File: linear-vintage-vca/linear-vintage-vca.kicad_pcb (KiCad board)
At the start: 2 copper layers, 50.5 x 110 mm, 51 parts, among them J1 Conn_02x08_Odd_Even, J2 AudioJack2, J3 AudioJack2, J4 AudioJack2, J5 AudioJack2, J6 AudioJack2, J7 AudioJack2, J8 AudioJack2, J9 AudioJack2, Q1 BC556, Q2 BC556, U1 LM13700, U2 TL072, U3 TL072

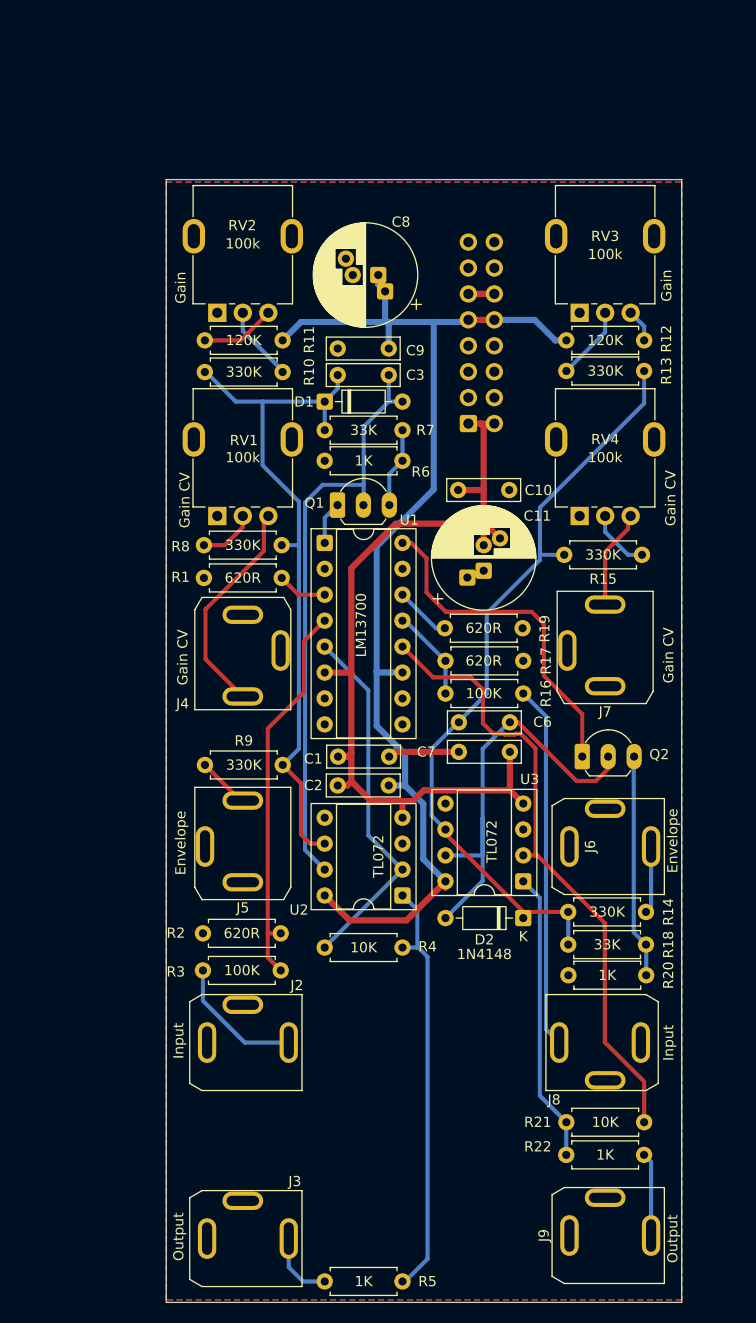
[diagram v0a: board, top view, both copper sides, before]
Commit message: VCA v. 2.0
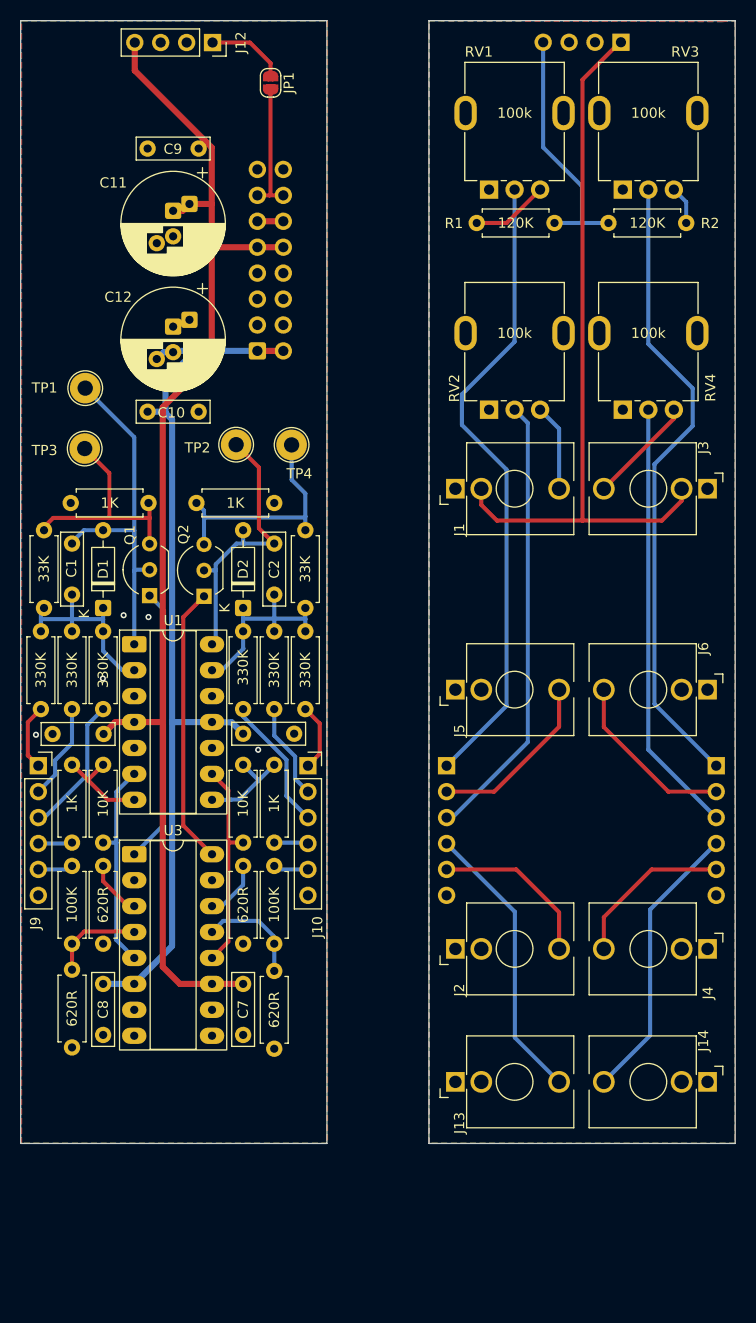
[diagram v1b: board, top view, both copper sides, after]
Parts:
- removed C3: 100n, Capacitor_THT:C_Rect_L7.0mm_W2.0mm_P5.00mm
- removed U2: TL072, Package_DIP:DIP-8_W7.62mm_Socket
- added C12: 47uF, Capacitor_THT:CP_Radial_D10.0mm_P2.50mm_P5.00mm, F.Cu at (50.7, 73.7)
- added C5: 100n, Capacitor_THT:C_Rect_L7.0mm_W2.0mm_P5.00mm, F.Cu at (43.9, 113.6)
- added J10: Conn_01x10_Socket, Connector_PinSocket_2.54mm:PinSocket_1x06_P2.54mm_Vertical, F.Cu at (63.9, 116.7)
- added J11: Conn_01x04_Pin, Connector_PinHeader_2.54mm:PinHeader_1x04_P2.54mm_Vertical, B.Cu at (94.5, 45.8)
- added J12: Conn_01x04_Socket, Connector_PinSocket_2.54mm:PinSocket_1x04_P2.54mm_Vertical, F.Cu at (54.5, 45.8)
- added J13: AudioJack2, linear_vintage_vca:Jack_3.5mm_Switch, F.Cu at (84.1, 147.6)
- added J14: AudioJack2, linear_vintage_vca:Jack_3.5mm_Switch, F.Cu at (97.2, 147.6)
- added J15: Conn_02x08_Odd_Even, Connector_IDC:IDC-Header_2x08_P2.54mm_Vertical, B.Cu at (58.9, 76.0)
- added JP1: SolderJumper_2_Open, Jumper:SolderJumper-2_P1.3mm_Open_RoundedPad1.0x1.5mm, F.Cu at (60.2, 49.8)
- added TP1: TestPoint, TestPoint:TestPoint_Loop_D2.54mm_Drill1.5mm_Beaded, F.Cu at (42.1, 79.7)
- added TP2: TestPoint, TestPoint:TestPoint_Loop_D2.54mm_Drill1.5mm_Beaded, F.Cu at (56.8, 85.2)
- added TP3: TestPoint, TestPoint:TestPoint_Loop_D2.54mm_Drill1.5mm_Beaded, F.Cu at (42.0, 85.6)
- added TP4: TestPoint, TestPoint:TestPoint_Loop_D2.54mm_Drill1.5mm_Beaded, F.Cu at (62.3, 85.2)
- C8: value 47uF -> 100n; footprint Capacitor_THT:CP_Radial_D10.0mm_P2.50mm_P5.00mm -> Capacitor_THT:C_Rect_L7.0mm_W2.0mm_P5.00mm
- J1: value Conn_02x08_Odd_Even -> AudioJack2; footprint Connector_IDC:IDC-Header_2x08_P2.54mm_Vertical -> linear_vintage_vca:Jack_3.5mm_Switch; moved to F.Cu
- J2, J3, J4, J5, J6: footprint linear_vintage_vca:Jack_3.5mm_PJ-341-2_Vertical -> linear_vintage_vca:Jack_3.5mm_Switch
- J7, J8: value AudioJack2 -> Conn_01x06_Pin; footprint linear_vintage_vca:Jack_3.5mm_PJ-341-2_Vertical -> Connector_PinHeader_2.54mm:PinHeader_1x06_P2.54mm_Vertical; moved to B.Cu
- J9: value AudioJack2 -> Conn_01x10_Socket; footprint linear_vintage_vca:Jack_3.5mm_PJ-341-2_Vertical -> Connector_PinSocket_2.54mm:PinSocket_1x06_P2.54mm_Vertical
- Q1, Q2: footprint linear_vintage_vca:TO-92_Inline_Wide -> Package_TO_SOT_THT:TO-92_Inline_Wide
- R1, R2: value 620R -> 120K
- R10, R9: value 330K -> 100K
- R11, R12: value 120K -> 620R
- R13, R14: value 330K -> 33K
- R15: value 330K -> 620R
- R16: value 100K -> 620R
- R17: value 620R -> 1K
- R18: value 33K -> 1K
- R19: value 620R -> 10K
- R20: value 1K -> 10K
- R21: value 10K -> 1K
- R3: value 100K -> 330K
- R4: value 10K -> 330K
- R5, R6: value 1K -> 330K
- R7: value 33K -> 330K
- U1: value LM13700 -> TL074; footprint Package_DIP:DIP-16_W7.62mm_Socket -> Package_DIP:DIP-14_W7.62mm_Socket_LongPads
- U3: value TL072 -> LM13700; footprint Package_DIP:DIP-8_W7.62mm_Socket -> Package_DIP:DIP-16_W7.62mm_Socket_LongPads
- moved J3 83.5 mm to (97.2, 89.5), turned to -90 degrees
- moved C8 79.2 mm to (43.8, 143.0), turned to 90 degrees
- moved R2 76.6 mm to (93.3, 63.5), turned to 0 degrees
- moved J9 72.1 mm to (37.5, 116.7), turned to 0 degrees
- moved R12 68.1 mm to (60.6, 136.8), turned to -90 degrees
- moved R21 66.1 mm to (40.8, 116.6), turned to -90 degrees
- moved R11 65.0 mm to (40.8, 136.7), turned to -90 degrees
- moved R5 63.3 mm to (43.8, 111.1), turned to 90 degrees
- moved R15 61.0 mm to (43.8, 126.5), turned to -90 degrees
- moved R18 56.6 mm to (53.0, 90.9)
- moved R13 56.2 mm to (38.0, 101.2), turned to 90 degrees
- moved J4 49.3 mm to (97.2, 134.6), turned to -90 degrees
- moved R10 48.4 mm to (60.6, 126.5), turned to -90 degrees
- moved R22 47.7 mm to (60.6, 116.6), turned to -90 degrees
- moved C11 46.6 mm to (50.7, 62.3), turned to -90 degrees
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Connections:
- C1 pad 1: +12V -> Net-(D1-K)
- C1 pad 2: -12V -> Net-(D1-A)
- C11 pad 1: GND -> +12V
- C11 pad 2: -12V -> GND
- C2 pad 1: +12V -> Net-(D2-K)
- C2 pad 2: -12V -> Net-(D2-A)
- C6 pad 1: Net-(D2-K) -> GND
- C6 pad 2: Net-(D2-A) -> -12V
- C7 pad 2: -12V -> GND
- C8 pad 1: +12V -> GND
- C8 pad 2: GND -> -12V
- J2 pad S: GND -> GND_A
- J2 pad T: Net-(J2-PadT) -> Net-(J7-Pin_5)
- J3 pad S: GND -> GND_A
- J4 pad S: GND -> GND_A
- J4 pad T: Net-(J4-PadT) -> Net-(J8-Pin_5)
- J5 pad S: GND -> GND_A
- J5 pad T: Net-(J5-PadT) -> Net-(J7-Pin_2)
- J6 pad S: GND -> GND_A
- J6 pad T: Net-(J6-PadT) -> Net-(J8-Pin_2)
- R1 pad 1: Net-(U1C-+) -> +12V_A
- R1 pad 2: GND -> Net-(R1-Pad2)
- R10 pad 1: Net-(R10-Pad1) -> Net-(J10-Pin_5)
- R10 pad 2: Net-(D1-K) -> Net-(U3A--)
- R11 pad 1: +12V -> Net-(U3C--)
- R11 pad 2: Net-(R11-Pad2) -> GND
- R12 pad 1: +12V -> Net-(U3A--)
- R12 pad 2: Net-(R12-Pad2) -> GND
- R13 pad 1: Net-(R13-Pad1) -> Net-(D1-K)
- R13 pad 2: Net-(D2-K) -> Net-(Q1-E)
- R14 pad 1: Net-(J6-PadT) -> Net-(D2-K)
- R14 pad 2: Net-(D2-K) -> Net-(Q2-E)
- R15 pad 1: Net-(R15-Pad1) -> Net-(U3C-+)
- R15 pad 2: Net-(D2-K) -> GND
- R16 pad 1: Net-(J8-PadT) -> Net-(U3A-+)
- R16 pad 2: Net-(U1A--) -> GND
- R17 pad 1: Net-(U1A--) -> Net-(Q1-E)
- R18 pad 1: Net-(D2-K) -> Net-(Q2-E)
- R18 pad 2: Net-(Q2-E) -> GND
- R19 pad 1: Net-(U1A-+) -> Net-(U1B--)
- R19 pad 2: GND -> Net-(R19-Pad2)
- R2 pad 1: Net-(U1C--) -> +12V_A
- R2 pad 2: GND -> Net-(R2-Pad2)
- R20 pad 1: Net-(Q2-E) -> Net-(U1C--)
- R20 pad 2: GND -> Net-(R20-Pad2)
- R21 pad 1: Net-(U3A--) -> Net-(R19-Pad2)
- R21 pad 2: Net-(R21-Pad2) -> OUT_1B
- R22 pad 1: Net-(R21-Pad2) -> Net-(R20-Pad2)
- R22 pad 2: Net-(J9-PadT) -> OUT_2B
- R3 pad 1: Net-(J2-PadT) -> Net-(J9-Pin_1)
- R3 pad 2: Net-(U1C--) -> Net-(D1-K)
- R4 pad 1: Net-(U2A--) -> Net-(J9-Pin_2)
- R4 pad 2: Net-(R4-Pad2) -> Net-(D1-K)
- R5 pad 1: Net-(R4-Pad2) -> Net-(J9-Pin_3)
- R5 pad 2: Net-(J3-PadT) -> Net-(D1-K)
- R6 pad 1: Net-(Q1-E) -> Net-(J10-Pin_1)
- R6 pad 2: GND -> Net-(D2-K)
- R7 pad 1: Net-(D1-K) -> Net-(J10-Pin_2)
- R7 pad 2: Net-(Q1-E) -> Net-(D2-K)
- R8 pad 1: Net-(R8-Pad1) -> Net-(J10-Pin_3)
- R8 pad 2: Net-(D1-K) -> Net-(D2-K)
- R9 pad 1: Net-(J5-PadT) -> Net-(J9-Pin_5)
- R9 pad 2: Net-(D1-K) -> Net-(U3C--)
- RV1 pad 1: GND -> GND_A
- RV1 pad 2: Net-(R8-Pad1) -> Net-(J7-Pin_1)
- RV1 pad 3: Net-(J4-PadT) -> Net-(R1-Pad2)
- RV2 pad 1: GND -> GND_A
- RV2 pad 2: Net-(R10-Pad1) -> Net-(J7-Pin_3)
- RV2 pad 3: Net-(R11-Pad2) -> Net-(J1-PadT)
- RV3 pad 1: GND -> GND_A
- RV3 pad 2: Net-(R13-Pad1) -> Net-(J8-Pin_1)
- RV3 pad 3: Net-(R12-Pad2) -> Net-(R2-Pad2)
- RV4 pad 1: GND -> GND_A
- RV4 pad 2: Net-(R15-Pad1) -> Net-(J8-Pin_3)
- RV4 pad 3: Net-(J7-PadT) -> Net-(J3-PadT)
- U1 pad 1: Net-(Q1-C) -> Net-(D1-A)
- U1 pad 11: +12V -> -12V
- U1 pad 12: Net-(U3A--) -> GND
- U1 pad 13: Net-(U1A--) -> Net-(D2-K)
- U1 pad 14: Net-(U1A-+) -> Net-(D2-A)
- U1 pad 2: unconnected-(U1C-DIODE_BIAS-Pad2) -> Net-(D1-K)
- U1 pad 3: Net-(U1C-+) -> GND
- U1 pad 4: Net-(U1C--) -> +12V
- U1 pad 5: Net-(U2A--) -> GND
- U1 pad 6: -12V -> Net-(U1B--)
- U1 pad 7: GND -> Net-(R19-Pad2)
- U1 pad 8: unconnected-(U1-Pad8) -> Net-(R20-Pad2)
- U1 pad 9: unconnected-(U1-Pad9) -> Net-(U1C--)
- U3 pad 1: Net-(R21-Pad2) -> Net-(Q1-C)
- U3 pad 2: Net-(U3A--) -> unconnected-(U3C-DIODE_BIAS-Pad2)
- U3 pad 3: GND -> Net-(U3C-+)
- U3 pad 4: -12V -> Net-(U3C--)
- U3 pad 5: GND -> Net-(U1B--)
- U3 pad 6: Net-(D2-K) -> -12V
- U3 pad 7: Net-(D2-A) -> unconnected-(U3-Pad7)
- U3 pad 8: +12V -> unconnected-(U3-Pad8)
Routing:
- net CV_A: track 0.00 -> 72.4 mm
- net Net-(J7-Pin_1): track 0.00 -> 63.5 mm
- net Net-(J8-Pin_1): track 0.00 -> 62.3 mm
- net Net-(D2-K): track 76.2 -> 20.0 mm
- net Net-(U3A--): track 61.5 -> 10.5 mm
- net Net-(D1-K): track 68.6 -> 20.0 mm
- net Net-(J7-Pin_3): track 0.00 -> 44.1 mm
- net Net-(J8-Pin_3): track 0.00 -> 42.7 mm
- net Net-(R4-Pad2): track 41.8 -> 0.00 mm
- net Net-(U2A--): track 35.8 -> 0.00 mm
- net Net-(J8-PadT): track 35.7 -> 0.00 mm
- net Net-(R21-Pad2): track 28.6 -> 0.00 mm
- net OUT_1A: track 0.00 -> 27.9 mm
- net OUT_2A: track 0.00 -> 27.9 mm
- net +12V_A: track 0.00 -> 24.7 mm
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- added copper zone on B.Cu, net GND_A
- added copper zone on F.Cu, net GND_A
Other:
- board size 50.5 x 110 mm -> 70 x 110 mm
- board text removed: "2025"
- board text removed: "Envelope"
- board text removed: "Gain"
- board text removed: "Gain CV"
- board text removed: "Input"
- board text removed: "Linear VCA"
- board text removed: "Output"
- board text removed: "ver. 1.2"
